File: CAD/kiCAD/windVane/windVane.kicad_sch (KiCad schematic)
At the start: 28 parts, among them J1 Conn_01x01, J2 Conn_01x01

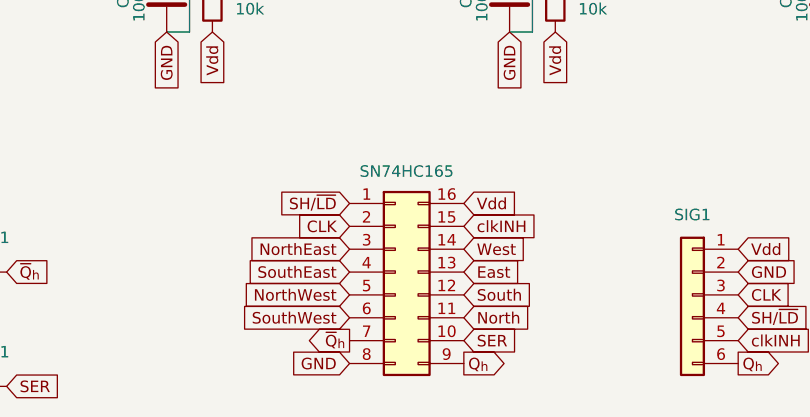
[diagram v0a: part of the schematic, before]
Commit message: Update
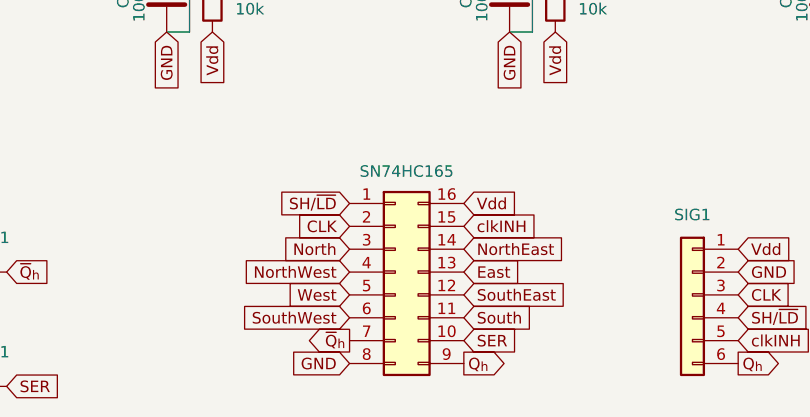
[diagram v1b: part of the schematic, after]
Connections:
- net North: now also SN74HC165.3 (Pin_3); no longer SN74HC165.11 (Pin_11)
- net NorthEast: now also SN74HC165.14 (Pin_14); no longer SN74HC165.3 (Pin_3)
- net NorthWest: now also SN74HC165.4 (Pin_4); no longer SN74HC165.5 (Pin_5)
- net South: now also SN74HC165.11 (Pin_11); no longer SN74HC165.12 (Pin_12)
- net SouthEast: now also SN74HC165.12 (Pin_12); no longer SN74HC165.4 (Pin_4)
- net West: now also SN74HC165.5 (Pin_5); no longer SN74HC165.14 (Pin_14)
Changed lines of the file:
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@@
 	(global_label "West"
 		(shape input)
-		(at 118.11 123.19 0)
-		(fields_autoplaced yes)
-		(effects
-			(font
-				(size 1.27 1.27)
-			)
-			(justify left)
-		)
-		(property "Intersheetrefs" "${INTERSHEET_REFS}"
-			(at 125.389 123.19 0)
-			(effects
-				(font
-					(size 1.27 1.27)
-				)
-				(justify left)
+		(at 105.41 128.27 180)
+		(fields_autoplaced yes)
+		(effects
+			(font
+				(size 1.27 1.27)
+			)
+			(justify right)
+		)
+		(property "Intersheetrefs" "${INTERSHEET_REFS}"
+			(at 98.131 128.27 0)
+			(effects
+				(font
+					(size 1.27 1.27)
+				)
+				(justify right)
 				(hide yes)
 			)
@@
 	(global_label "South"
 		(shape input)
-		(at 118.11 128.27 0)
-		(fields_autoplaced yes)
-		(effects
-			(font
-				(size 1.27 1.27)
-			)
-			(justify left)
-		)
-		(property "Intersheetrefs" "${INTERSHEET_REFS}"
-			(at 126.4774 128.27 0)
+		(at 118.11 130.81 0)
+		(fields_autoplaced yes)
+		(effects
+			(font
+				(size 1.27 1.27)
+			)
+			(justify left)
+		)
+		(property "Intersheetrefs" "${INTERSHEET_REFS}"
+			(at 126.4774 130.81 0)
 			(effects
 				(font
@@
 	(global_label "North"
 		(shape input)
-		(at 118.11 130.81 0)
-		(fields_autoplaced yes)
-		(effects
-			(font
-				(size 1.27 1.27)
-			)
-			(justify left)
-		)
-		(property "Intersheetrefs" "${INTERSHEET_REFS}"
-			(at 126.2356 130.81 0)
-			(effects
-				(font
-					(size 1.27 1.27)
-				)
-				(justify left)
+		(at 105.41 123.19 180)
+		(fields_autoplaced yes)
+		(effects
+			(font
+				(size 1.27 1.27)
+			)
+			(justify right)
+		)
+		(property "Intersheetrefs" "${INTERSHEET_REFS}"
+			(at 97.2844 123.19 0)
+			(effects
+				(font
+					(size 1.27 1.27)
+				)
+				(justify right)
 				(hide yes)
 			)
@@
 	(global_label "NorthWest"
 		(shape input)
-		(at 105.41 128.27 180)
-		(fields_autoplaced yes)
-		(effects
-			(font
-				(size 1.27 1.27)
-			)
-			(justify right)
-		)
-		(property "Intersheetrefs" "${INTERSHEET_REFS}"
-			(at 92.9906 128.27 0)
+		(at 105.41 125.73 180)
+		(fields_autoplaced yes)
+		(effects
+			(font
+				(size 1.27 1.27)
+			)
+			(justify right)
+		)
+		(property "Intersheetrefs" "${INTERSHEET_REFS}"
+			(at 92.9906 125.73 0)
 			(effects
 				(font
@@
 	(global_label "NorthEast"
 		(shape input)
-		(at 105.41 123.19 180)
-		(fields_autoplaced yes)
-		(effects
-			(font
-				(size 1.27 1.27)
-			)
-			(justify right)
-		)
-		(property "Intersheetrefs" "${INTERSHEET_REFS}"
-			(at 93.2326 123.19 0)
-			(effects
-				(font
-					(size 1.27 1.27)
-				)
-				(justify right)
+		(at 118.11 123.19 0)
+		(fields_autoplaced yes)
+		(effects
+			(font
+				(size 1.27 1.27)
+			)
+			(justify left)
+		)
+		(property "Intersheetrefs" "${INTERSHEET_REFS}"
+			(at 130.2874 123.19 0)
+			(effects
+				(font
+					(size 1.27 1.27)
+				)
+				(justify left)
 				(hide yes)
 			)
@@
 	(global_label "SouthEast"
 		(shape input)
-		(at 105.41 125.73 180)
-		(fields_autoplaced yes)
-		(effects
-			(font
-				(size 1.27 1.27)
-			)
-			(justify right)
-		)
-		(property "Intersheetrefs" "${INTERSHEET_REFS}"
-			(at 92.9908 125.73 0)
-			(effects
-				(font
-					(size 1.27 1.27)
-				)
-				(justify right)
-				(hide yes)
-			)
+		(at 118.11 128.27 0)
+		(fields_autoplaced yes)
+		(effects
+			(font
+				(size 1.27 1.27)
+			)
+			(justify left)
+		)
+		(property "Intersheetrefs" "${INTERSHEET_REFS}"
+			(at 130.5292 128.27 0)
+			(effects
+				(font
+					(size 1.27 1.27)
+				)
+				(justify left)
+				(hide yes)
+			)
